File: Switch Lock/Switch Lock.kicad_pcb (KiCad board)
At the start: 2 copper layers, 40.2 x 26.2 mm, 10 parts, among them J2 Conn_01x07

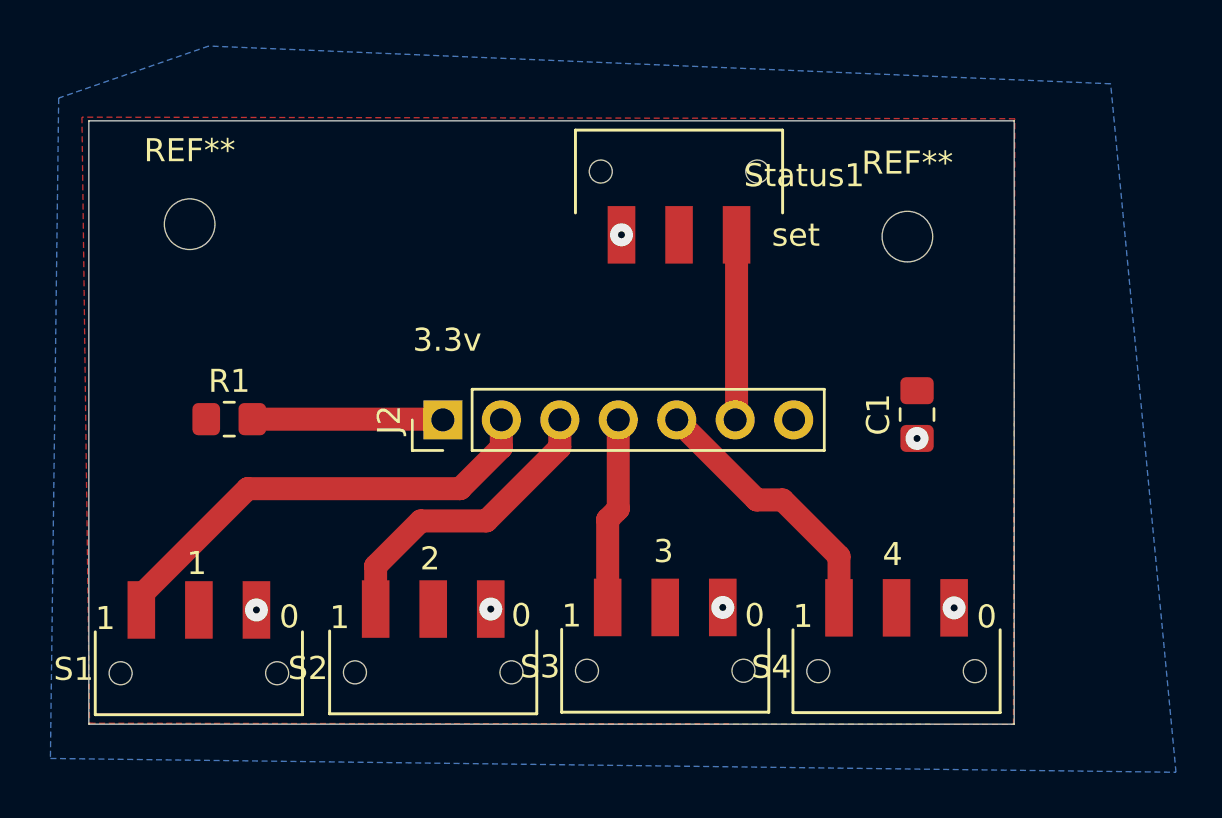
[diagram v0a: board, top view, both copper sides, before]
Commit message: 3dmodoling
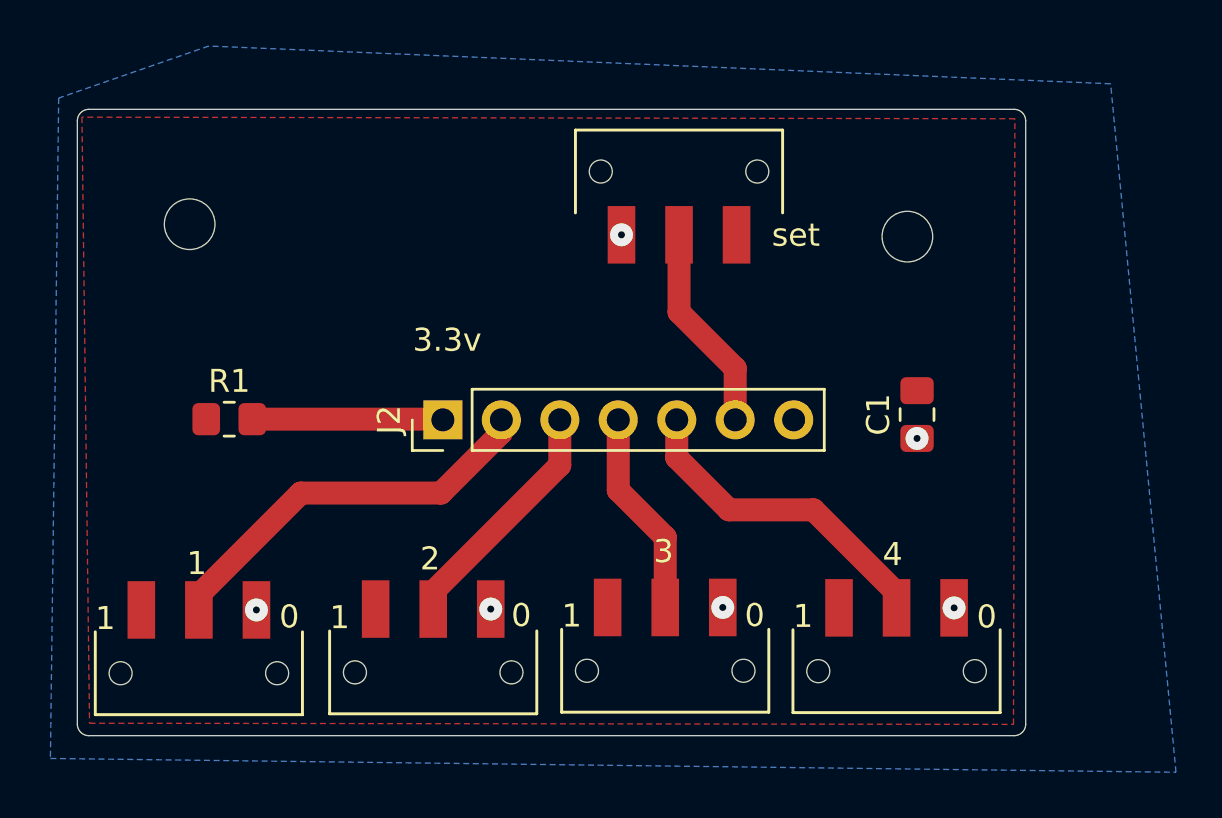
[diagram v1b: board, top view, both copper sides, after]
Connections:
- S1 pad 1: Net-(J2-Pin_2) -> /3.3v
- S1 pad 2: /3.3v -> Net-(J2-Pin_2)
- S2 pad 1: Net-(J2-Pin_3) -> /3.3v
- S2 pad 2: /3.3v -> Net-(J2-Pin_3)
- S3 pad 1: Net-(J2-Pin_4) -> /3.3v
- S3 pad 2: /3.3v -> Net-(J2-Pin_4)
- S4 pad 1: Net-(J2-Pin_5) -> /3.3v
- S4 pad 2: /3.3v -> Net-(J2-Pin_5)
- Status1 pad 1: Net-(J2-Pin_6) -> /3.3v
- Status1 pad 2: /3.3v -> Net-(J2-Pin_6)
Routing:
- net Net-(J2-Pin_2): track 20.1 -> 17.3 mm
- net Net-(J2-Pin_3): track 13.2 -> 10.5 mm
- net Net-(J2-Pin_5): track 11.7 -> 14.3 mm
- net Net-(J2-Pin_6): track 8.06 -> 9.05 mm
- net Net-(J2-Pin_4): track 8.34 -> 8.99 mm
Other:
- board size 40.2 x 26.2 mm -> 41.2 x 27.2 mm
